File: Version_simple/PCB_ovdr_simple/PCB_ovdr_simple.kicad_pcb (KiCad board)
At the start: 2 copper layers, 79.4 x 63.5 mm, 42 parts, among them J1 Input, J2 Output, J3 Vcc, J5 Out_Auri, U1 TL072, U2 TL072, U3 LM386

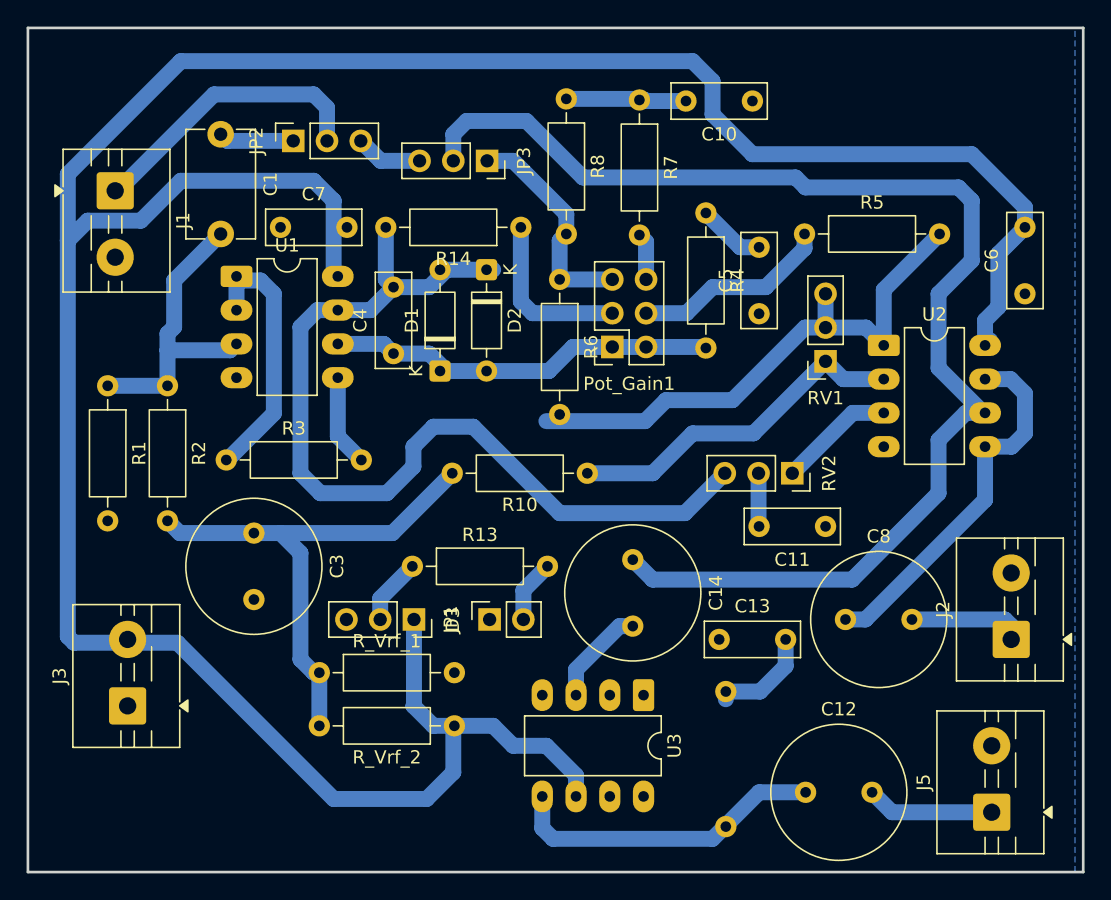
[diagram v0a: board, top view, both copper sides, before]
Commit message: update
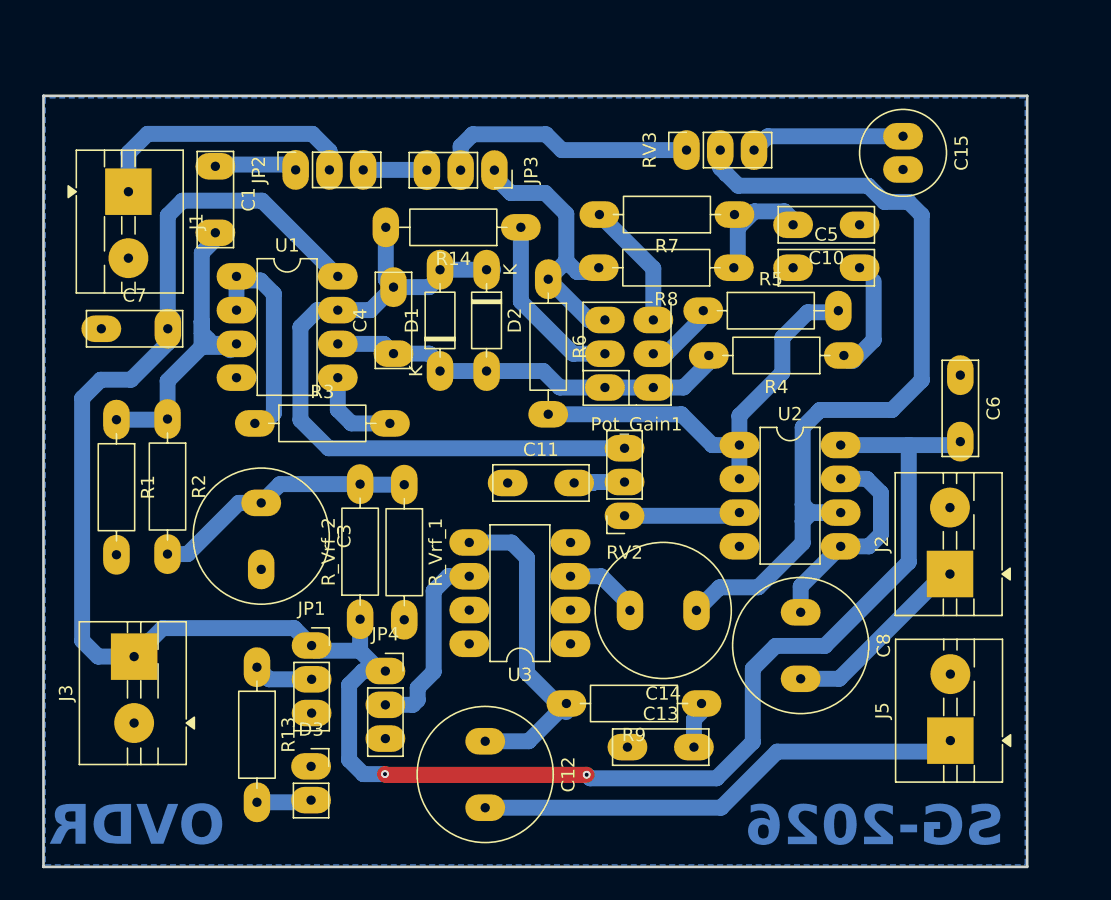
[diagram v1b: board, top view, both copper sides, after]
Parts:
- removed R10: R_US, Resistor_THT:R_Axial_DIN0207_L6.3mm_D2.5mm_P10.16mm_Horizontal
- removed RV1: Pot_vol, Connector_PinSocket_2.54mm:PinSocket_1x03_P2.54mm_Vertical
- added C15: C_Polarized, Capacitor_THT:C_Radial_D6.3mm_H5.0mm_P2.50mm, F.Cu at (170.8, 87.2)
- added JP4: FootSW_2, Connector_PinSocket_2.54mm:PinSocket_1x03_P2.54mm_Vertical, F.Cu at (131.9, 127.4)
- added RV3: Pot_vol, Connector_PinSocket_2.54mm:PinSocket_1x03_P2.54mm_Vertical, F.Cu at (154.5, 88.2)
- C1: footprint Capacitor_THT:C_Disc_D8.0mm_W5.0mm_P7.50mm -> Capacitor_THT:C_Disc_D7.0mm_W2.5mm_P5.00mm
- R9: moved to F.Cu
- moved C12 24.4 mm to (139.4, 132.7), turned to -90 degrees
- moved C11 24.1 mm to (141.1, 113.2), turned to 0 degrees
- moved R8 17.9 mm to (158.1, 97.0), turned to 180 degrees
- moved D3 17.4 mm to (126.3, 134.6), turned to 0 degrees
- moved R_Vrf_1 15.5 mm to (133.3, 113.4), turned to -90 degrees
- moved C7 15.5 mm to (110.5, 101.6)
- moved R4 14.9 mm to (166.4, 103.6), turned to 180 degrees
- moved R13 13.9 mm to (122.2, 127.1), turned to -90 degrees
- moved U2 13.2 mm to (158.5, 110.4)
- moved RV2 13.0 mm to (149.9, 115.7), turned to 180 degrees
- moved C10 12.3 mm to (167.6, 93.8)
- moved R7 11.2 mm to (158.2, 93.0), turned to 180 degrees
- moved R_Vrf_2 10.7 mm to (130.0, 123.5), turned to 90 degrees
- moved C13 10.6 mm to (150.1, 133.1)
- moved R5 9.56 mm to (155.8, 100.3)
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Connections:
- C14 pad 1: Net-(JP3-C) -> Net-(U2B--)
- R5 pad 2: Net-(R5-Pad2) -> Net-(U2A--)
- R6 pad 2: Net-(R5-Pad2) -> Net-(U2A--)
- U2 pad 1: Net-(R5-Pad2) -> Net-(U2A--)
- U2 pad 6: Net-(JP3-C) -> Net-(U2B--)
- U3 pad 6: /9V -> Net-(JP4-C)
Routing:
- net Net-(JP3-C): track 97.1 -> 19.6 mm
- net Net-(U2B--): track 0.00 -> 65.9 mm
- net /9V: track 217.7 -> 159.2 mm, vias 0 -> 2
- net Net-(R5-Pad2): track 41.5 -> 0.00 mm
- net Net-(J5-Pin_1): track 9.62 -> 37.1 mm
- net /V_ref: track 39.6 -> 20.0 mm
- net Net-(D1-A): track 71.5 -> 53.3 mm
- net Net-(JP4-C): track 0.00 -> 15.3 mm
- net Net-(U2B-+): track 28.1 -> 16.2 mm
- net Net-(C15-Pad1): track 0.00 -> 11.6 mm
- net Net-(Pot_Gain1-Pad4): track 15.0 -> 5.81 mm
- net Net-(U1A-+): track 23.0 -> 29.8 mm
- net Net-(Pot_Gain1-Pad6): track 3.55 -> 9.61 mm
- net Net-(U2A--): track 26.3 -> 32.4 mm
- net Net-(J2-Pin_1): track 8.69 -> 14.5 mm
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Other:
- board size 79.4 x 63.5 mm -> 74 x 58 mm
- board text added: "OVDR"
- board text added: "SG-2026"
